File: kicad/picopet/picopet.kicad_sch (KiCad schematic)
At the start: 32 parts, among them J1 Conn_01x14_Pin, J2 Conn_01x02_Socket, J3 Conn_01x02_Socket, J4 Conn_01x02_Socket, J5 USB_C_Receptacle_USB2.0_14P, M1 Motor_DC, SW1 SW_SPST, SW2 SW_Push, SW3 SW_Push, SW4 SW_Push, SW5 SW_Push, SW6 SW_Push, SW7 SW_Push, U1 RP2040, U2 W25Q32JVSS, U3 MCP73831-2-MC, U4 DS3231MZ, U5 BQ27427YZFR, U6 AT24CS32-SSHM, U8 XC6206PxxxMR, Y1 ASCO

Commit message: Updating schematics
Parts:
- removed BT1: RTC_Battery 3V, symbol Device:Battery_Cell
- removed BT2: Single Li-Ion Cell, symbol Device:Battery_Cell
- removed C2, C3: 1uF, symbol Device:C
- removed C4: 2.2uF, symbol Device:C
- removed J2, J3, J4: Conn_01x02_Socket, symbol Connector:Conn_01x02_Socket
- removed R10, R9: 5.1k, symbol Device:R
- removed R11, R12: 10k, symbol Device:R
- removed R8: 2K, symbol Device:R
- removed SW7: SW_Push, symbol Switch:SW_Push
- removed U1: RP2040, Package_DFN_QFN:QFN-56-1EP_7x7mm_P0.4mm_EP3.2x3.2mm, symbol MCU_RaspberryPi:RP2040
- removed U2: W25Q32JVSS, Package_SO:SOIC-8_5.3x5.3mm_P1.27mm, symbol Memory_Flash:W25Q32JVSS
- removed U3: MCP73831-2-MC, Package_DFN_QFN:DFN-8-1EP_3x2mm_P0.5mm_EP1.7x1.4mm, symbol Battery_Management:MCP73831-2-MC
- removed U5: BQ27427YZFR, DSBGA9-YZF_TEX, symbol 2025-03-19_04-45-52:BQ27427YZFR
- removed U8: XC6206PxxxMR, Package_TO_SOT_SMD:SOT-23-3, symbol Regulator_Linear:XC6206PxxxMR
- removed Y1: ASCO, Oscillator:Oscillator_SMD_Abracon_ASCO-4Pin_1.6x1.2mm, symbol Oscillator:ASCO
- added C1, C10, C12, C13, C16, C19, C5, C6, C7, C8: 100n, Capacitor_SMD:C_0402_1005Metric, symbol Device:C
- added C11, C9: 1u, Capacitor_SMD:C_0402_1005Metric, symbol Device:C
- added C14, C15: 4.7u, Capacitor_SMD:C_0805_2012Metric, symbol Device:C
- added C17, C18: 1u, Capacitor_SMD:C_0805_2012Metric, symbol Device:C
- added C20, C21: 27p, Capacitor_SMD:C_0402_1005Metric, symbol Device:C
- added J2: MicroJST 1.25mm female, Connector_JST:JST_GH_SM02B-GHS-TB_1x02-1MP_P1.25mm_Horizontal, symbol Connector_Generic:Conn_01x02
- added J3: CR1220 Holder, Battery:BatteryHolder_LINX_BAT-HLD-012-SMT, symbol Connector_Generic:Conn_01x02
- added R1, R13, R14, R15, R2, R5, R6, R7: 5.1k, symbol Device:R
- added R16, R18: 1k, Capacitor_SMD:C_0402_1005Metric, symbol Device:R
- added R17: DNF, Capacitor_SMD:C_0402_1005Metric, symbol Device:R
- added R3, R4: 27, Capacitor_SMD:C_0402_1005Metric, symbol Device:R
- added U1: RP2040, RP2040_minimal:RP2040-QFN-56, symbol MCU_RaspberryPi_RP2040:RP2040
- added U2: MCP73831-2-OT, Package_TO_SOT_SMD:SOT-23-5, symbol Battery_Management:MCP73831-2-OT
- added U3: S-T111B33MC-OGSTFU, Package_TO_SOT_SMD:SOT-23-5, symbol Regulator_Linear:TPS77012PDBV
- added U7: W25Q128JVS, Package_SO:SOIC-8_5.23x5.23mm_P1.27mm, symbol RP2040_minimal-rescue:W25Q128JVS-Memory_Flash
- added Y1: ABLS-12.000MHZ-B4-T, RP2040_minimal:Crystal_SMD_HC49-US, symbol Device:Crystal
- SW1: value SW_SPST -> PWR
- SW2: renamed from SW6; value SW_Push -> BOOTSEL
- SW4: renamed from SW2; value SW_Push -> Btn0
- SW5: renamed from SW3; value SW_Push -> Btn1
- SW6: renamed from SW4; value SW_Push -> Btn2
- SW7: renamed from SW5; value SW_Push -> Btn3
- renumbered J5 to J1, J1 to J4
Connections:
- net GND: now also J1.A1 (GND), J1.A12 (GND), J1.B1 (GND), J1.B12 (GND), J1.S1 (SHIELD), SW2.1, U4.5 (GND), U6.1 (A0), U6.2 (A1), U6.3 (A2), U6.4 (GND), U6.7 (WP), C1.2, C10.2, C11.2, C12.2, C13.2, C14.2, C15.2, C16.2, C17.2, C18.2, C19.2, C20.2, C21.2, C5.2, C6.2, C7.2, C8.2, C9.2, J2.2 (Pin_2), J3.2 (Pin_2), R1.2, R2.2, R5.1, U1.19 (TESTEN), U1.57 (GND), U2.2 (V_{SS}), U3.2 (GND), U3.4 (GND), U7.4 (GND)
- net VBAT: now also SW1.1 (A), C15.1, J2.1 (Pin_1), U2.3 (V_{BAT})
- net GPIO_0: now reaches U6.5 (SDA)
- net GPIO_0: now also U4.7 (SDA), R15.1, R7.1
- net GPIO_1: now reaches U6.6 (SCL)
- net GPIO_1: now also U4.8 (SCL), R14.1, R6.1
- net +3V3: now reaches U6.8 (VCC)
- net +3V3: now also U4.2 (VCC), C1.1, C10.1, C16.1, C17.1, C19.1, C5.1, C6.1, C7.1, C8.1, C9.1, R13.2, R14.2, R15.2, R17.1, R6.2, R7.2, U1.1 (IOVDD), U1.10 (IOVDD), U1.22 (IOVDD), U1.33 (IOVDD), U1.42 (IOVDD), U1.43 (ADC_AVDD), U1.44 (VREG_IN), U1.48 (USB_VDD), U1.49 (IOVDD), U3.5 (OUT), U7.8 (VCC)
- net GPIO_5: now reaches U4.3 (~{INT}/SQW)
- net GPIO_5: now also R13.1
- net VCOIN: now reaches U4.6 (VBAT)
- net VCOIN: now also J3.1 (Pin_1)
- net at SW2.2: now also R16.2
- net at J1.A4 (VBUS), J1.A9 (VBUS), J1.B4 (VBUS)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: now also C14.1, U2.4 (V_{DD})
- net at J1.A5 (CC1): now also R1.1
- net USB_D+: now reaches J1.A6 (D+)
- net USB_D+: now also J1.B6 (D+), R3.1
- net USB_D-: now reaches J1.A7 (D-)
- net USB_D-: now also J1.B7 (D-), R4.1
- net at J1.B5 (CC2): now also R2.1
- net at SW1.2 (B): now also C18.1, U3.1 (IN), U3.3 (EN)
- new net: R3.2, U1.47 (USB_DP)
- new net: R4.2, U1.46 (USB_DM)
- new net: C21.1, R18.2, Y1.2
- new net: R5.2, U2.5 (PROG)
- new net +1V1: C11.1, C12.1, C13.1, U1.23 (DVDD), U1.45 (VREG_VOUT), U1.50 (DVDD)
- new net GPIO0: U1.2 (GPIO0)
- new net GPIO1: U1.3 (GPIO1)
- new net GPIO10: U1.13 (GPIO10)
- new net GPIO11: U1.14 (GPIO11)
- new net GPIO12: U1.15 (GPIO12)
- new net GPIO13: U1.16 (GPIO13)
- new net GPIO14: U1.17 (GPIO14)
- new net GPIO15: U1.18 (GPIO15)
- new net GPIO16: U1.27 (GPIO16)
- new net GPIO17: U1.28 (GPIO17)
- new net GPIO18: U1.29 (GPIO18)
- new net GPIO19: U1.30 (GPIO19)
- new net GPIO2: U1.4 (GPIO2)
- new net GPIO20: U1.31 (GPIO20)
- new net GPIO21: U1.32 (GPIO21)
- new net GPIO22: U1.34 (GPIO22)
- new net GPIO23: U1.35 (GPIO23)
- new net GPIO24: U1.36 (GPIO24)
- new net GPIO25: U1.37 (GPIO25)
- new net GPIO26_ADC0: U1.38 (GPIO26_ADC0)
- new net GPIO27_ADC1: U1.39 (GPIO27_ADC1)
- new net GPIO28_ADC2: U1.40 (GPIO28_ADC2)
- new net GPIO29_ADC3: U1.41 (GPIO29_ADC3)
- new net GPIO3: U1.5 (GPIO3)
- new net GPIO4: U1.6 (GPIO4)
- new net GPIO5: U1.7 (GPIO5)
- new net GPIO6: U1.8 (GPIO6)
- new net GPIO7: U1.9 (GPIO7)
- new net GPIO8: U1.11 (GPIO8)
- new net GPIO9: U1.12 (GPIO9)
- new net GPIO_UNDECIDED: U2.1 (STAT)
- new net QSPI_SCLK: U1.52 (QSPI_SCLK), U7.6 (CLK)
- new net QSPI_SD0: U1.53 (QSPI_SD0), U7.5 (DI(IO0))
- new net QSPI_SD1: U1.55 (QSPI_SD1), U7.2 (DO(IO1))
- new net QSPI_SD2: U1.54 (QSPI_SD2), U7.3 (IO2)
- new net QSPI_SD3: U1.51 (QSPI_SD3), U7.7 (IO3)
- new net QSPI_SS: R16.1, R17.2, U1.56 (QSPI_SS), U7.1 (~{CS})
- new net RUN: U1.26 (RUN)
- new net SWCLK: U1.24 (SWCLK)
- new net SWD: U1.25 (SWD)
- new net XIN: C20.1, U1.20 (XIN), Y1.1
- new net XOUT: R18.1, U1.21 (XOUT)
- no-connect marks 0 -> 2
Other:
- note added: "Make sure C11 is close to pin 45 of RP2040"
- note added: "Make sure C9 is close to pin 44 of RP2040"
- note added: "Make sure R3 and R4 are close to RP2040"
- moved on the sheet: BZ1, J1, J4, M1, SW1, SW2, SW4, SW5, SW6, SW7, U4

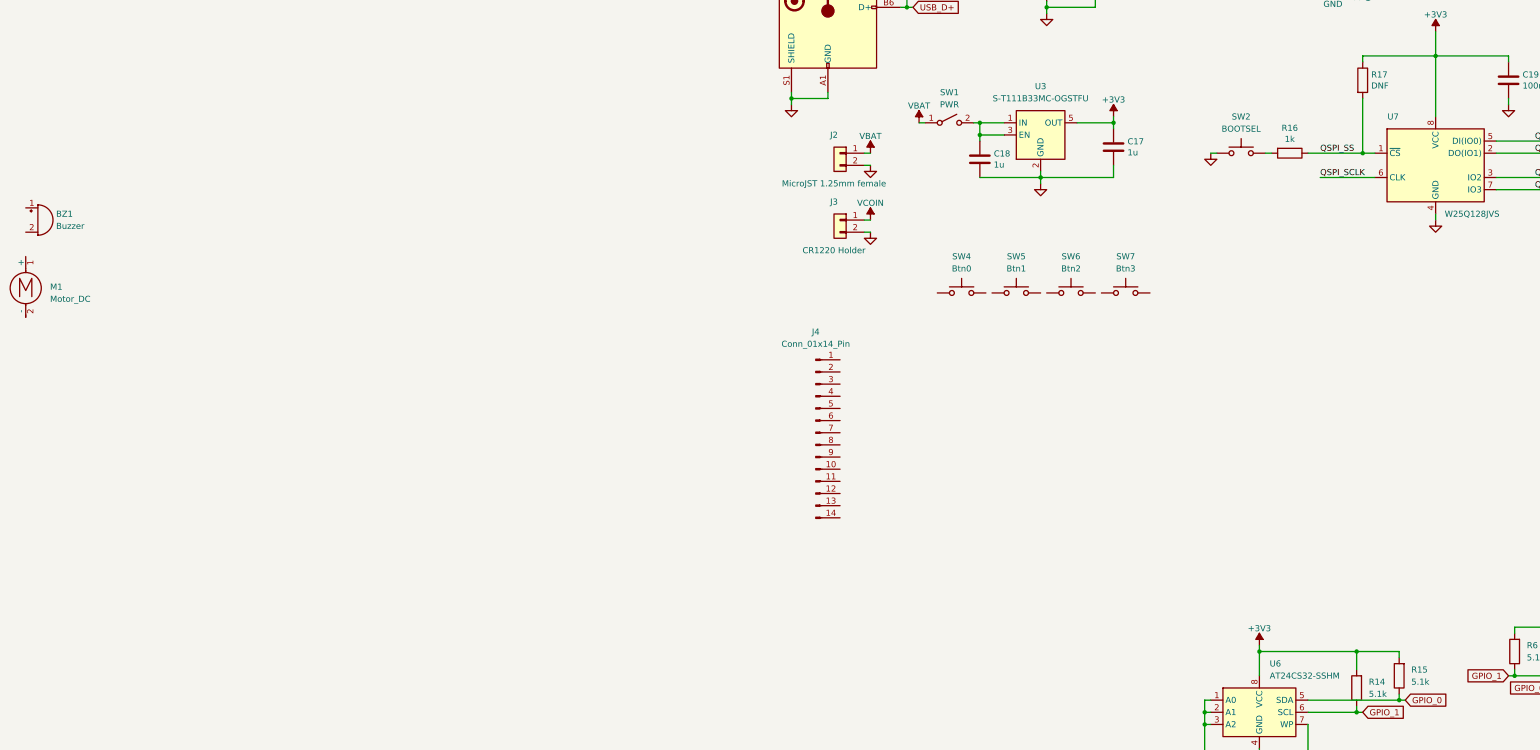
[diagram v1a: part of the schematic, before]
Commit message: More schematic work
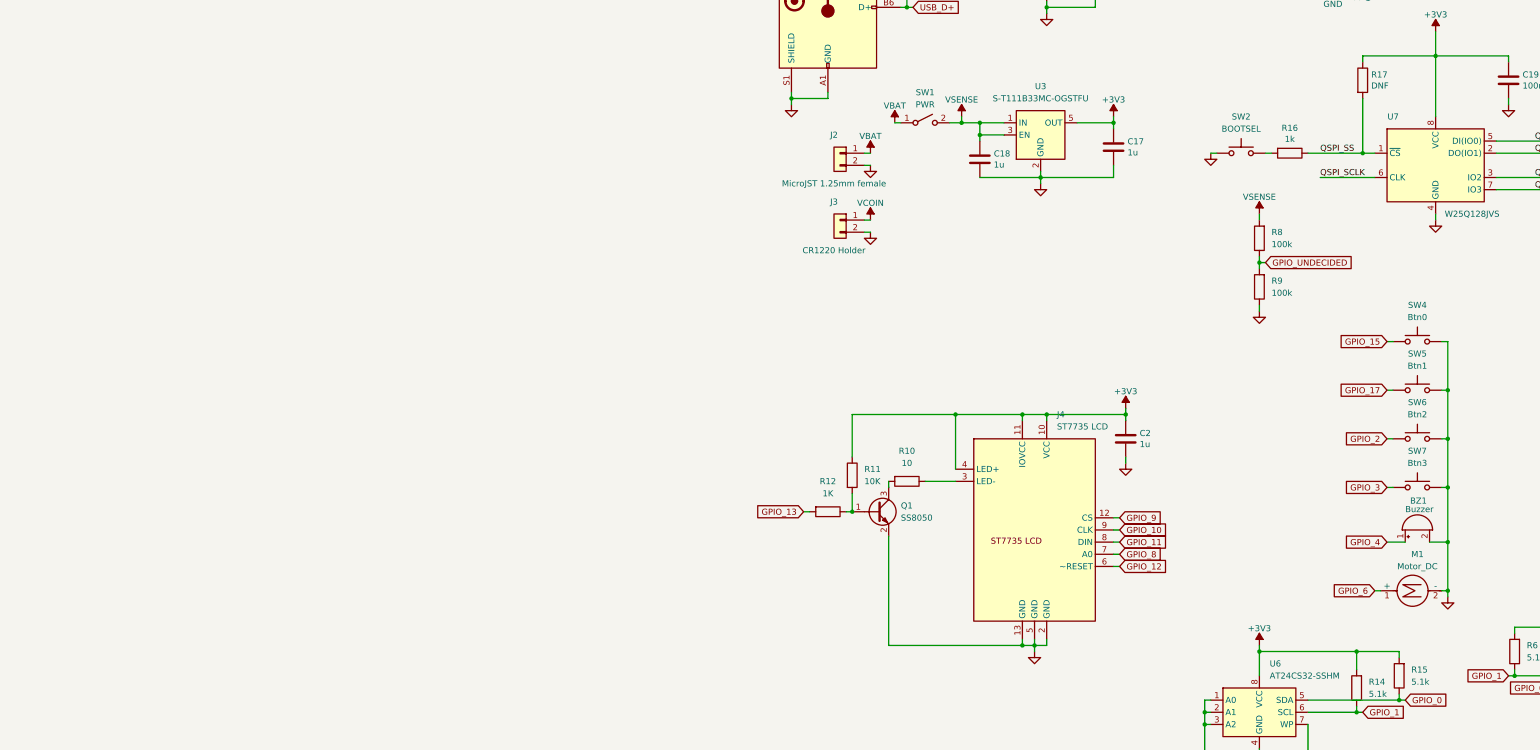
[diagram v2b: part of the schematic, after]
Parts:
- removed J4: Conn_01x14_Pin, symbol Connector:Conn_01x14_Pin
- added C2: 1u, Capacitor_SMD:C_0805_2012Metric, symbol Device:C
- added J4: ST7735 LCD, custom:ST7735_P0.8mm, symbol custom:ST7735
- added Q1: SS8050, Package_TO_SOT_SMD:SOT-23, symbol Transistor_BJT:SS8050
- added R10: 10, symbol Device:R
- added R11: 10K, symbol Device:R
- added R12: 1K, symbol Device:R
- added R8, R9: 100k, symbol Device:R
- BZ1: footprint (none) -> Buzzer_Beeper:MagneticBuzzer_CUI_CMT-8504-100-SMT
- J1: footprint (none) -> Connector_USB:USB_C_Receptacle_G-Switch_GT-USB-7025
- M1: footprint (none) -> Connector_JST:JST_GH_SM02B-GHS-TB_1x02-1MP_P1.25mm_Horizontal
- SW1: footprint (none) -> Button_Switch_THT:SW_Slide_SPDT_Angled_CK_OS102011MA1Q
- SW4, SW5, SW6, SW7: footprint (none) -> Button_Switch_SMD:SW_SPST_EVQP2_MiddlePushTravel_H2.5mm
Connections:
- net +3V3: now also C2.1, J4.10 (VCC), J4.11 (IOVCC), J4.4 (LED+), R11.1
- net GND: now also BZ1.2 (-), M1.2 (-), SW4.2, SW5.2, SW6.2, SW7.2, C2.2, J4.13 (GND), J4.2 (GND), J4.5 (GND), Q1.2 (E), R9.1
- net GPIO_UNDECIDED: now also R8.1, R9.2
- net GPIO_6: now reaches M1.1 (+)
- net GPIO_15: now reaches SW4.1
- net GPIO_4: now reaches BZ1.1 (+)
- net GPIO_2: now reaches SW6.1
- net VSENSE: now reaches C18.1, SW1.2 (B), U3.1 (IN), U3.3 (EN)
- net VSENSE: now also R8.2
- net GPIO_3: now reaches SW7.1
- net GPIO_17: now reaches SW5.1
- new net: Q1.1 (B), R11.2, R12.1
- new net: J4.3 (LED-), R10.1
- new net: Q1.3 (C), R10.2
- new net GPIO_10: J4.9 (CLK)
- new net GPIO_11: J4.8 (DIN)
- new net GPIO_12: J4.6 (~RESET)
- new net GPIO_13: R12.2
- new net GPIO_8: J4.7 (A0)
- new net GPIO_9: J4.12 (CS)
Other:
- moved on the sheet: BZ1, M1, SW1, SW4, SW5, SW6, SW7
